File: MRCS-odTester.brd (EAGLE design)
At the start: 50 x 50 mm, 14 parts

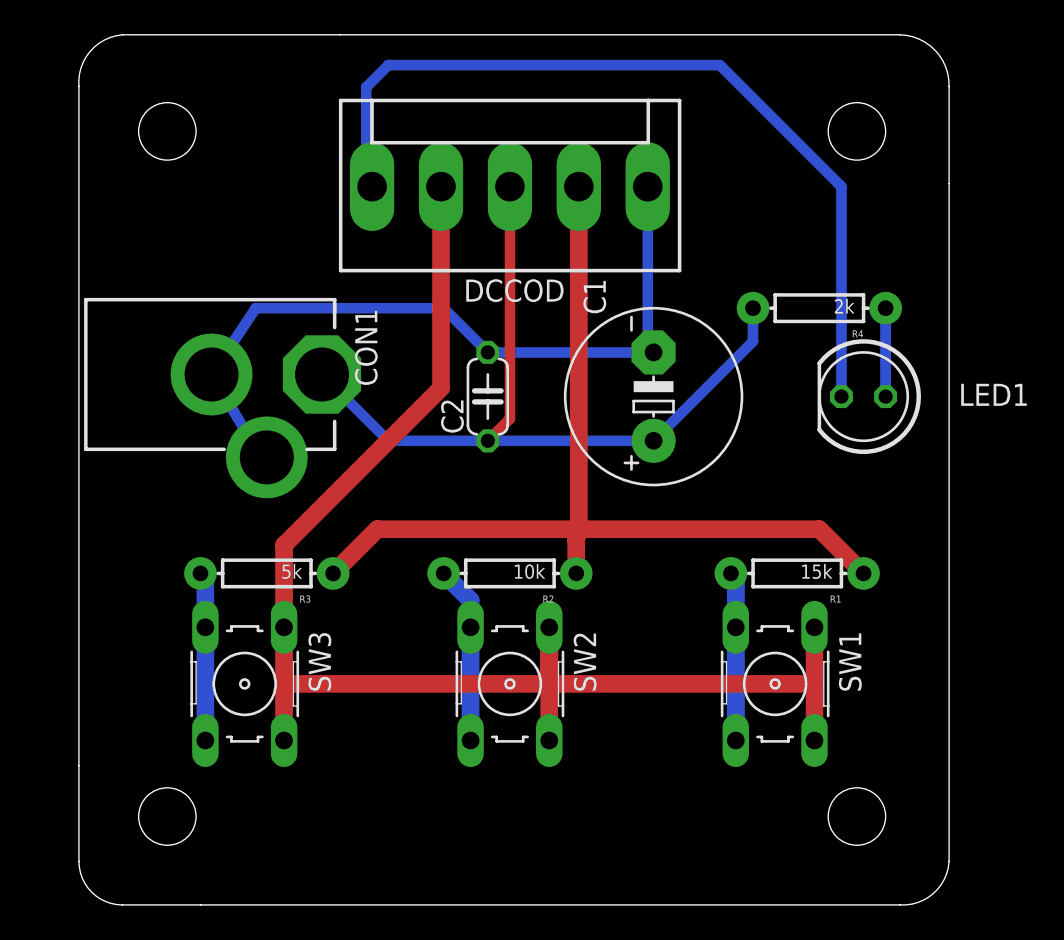
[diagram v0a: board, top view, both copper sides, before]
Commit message: 1.1
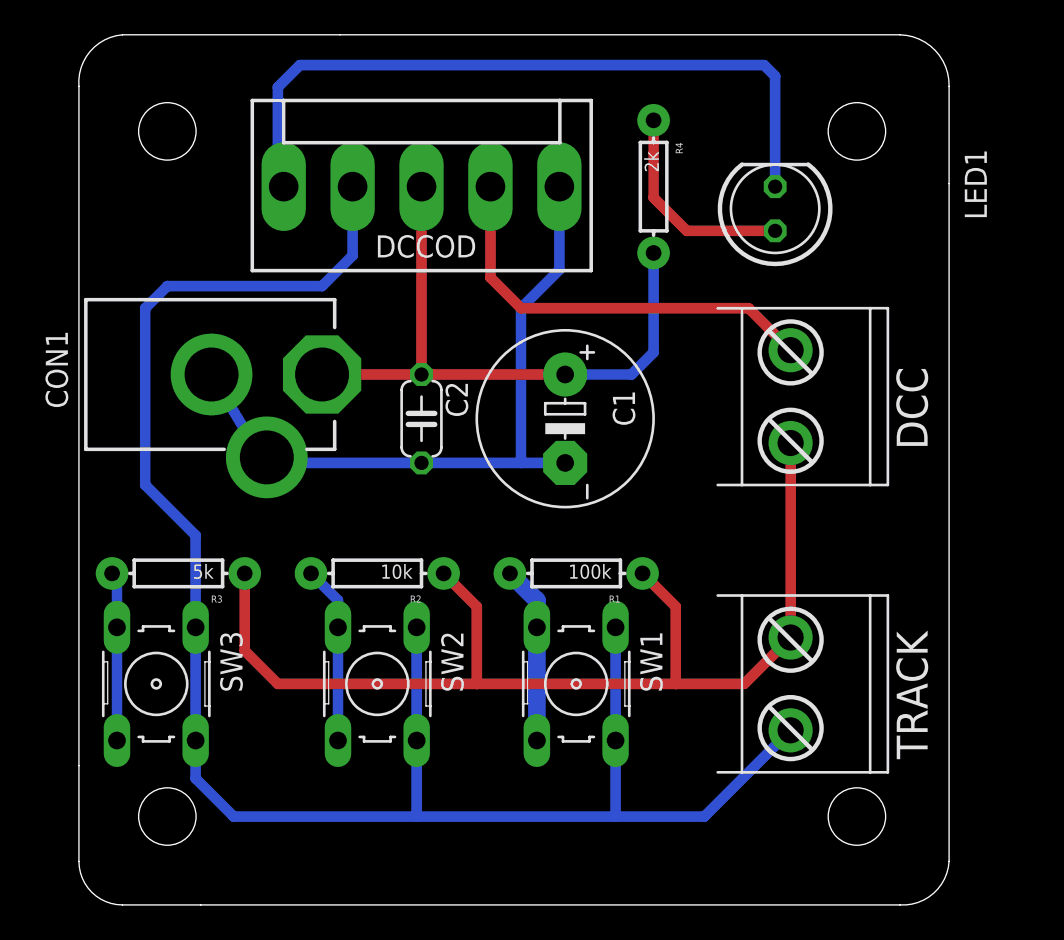
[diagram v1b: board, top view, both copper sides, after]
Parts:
- added DCC, TRACK: (no value), SPCoast:MSTB2
- R1: value 15k -> 100k
- moved R1 12.7 mm to (28.6, 19.1)
- moved LED1 11.9 mm to (40.0, 40.0), turned to 90 degrees
- moved R4 11.8 mm to (33.0, 41.3), turned to 270 degrees
- moved SW1 11.4 mm to (28.6, 12.7)
- moved R2 7.62 mm to (17.1, 19.1)
- moved SW2 7.62 mm to (17.1, 12.7)
- moved C1 5.24 mm to (27.9, 27.9), turned to 270 degrees
- moved DCCOD 5.08 mm to (19.7, 41.3)
- moved R3 5.08 mm to (5.71, 19.1)
- moved SW3 5.08 mm to (4.45, 12.7)
- moved C2 4.02 mm to (19.7, 27.9), turned to 270 degrees
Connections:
- removed net TRACK+: DCCOD.2, SW1.1, SW1.2, SW2.1, SW2.2, SW3.1, SW3.2
- removed net TRACK-: DCCOD.4, R1.P$1, R2.P$1, R3.P$1
- new net DCC-COMMON: DCC.2, DCCOD.4
- new net DCC-FROMTRACK: DCCOD.2, SW1.1, SW1.2, SW2.1, SW2.2, SW3.1, SW3.2, TRACK.1
- new net DCC-TOTRACK: DCC.1, R1.P$1, R2.P$1, R3.P$1, TRACK.2
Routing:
- net DCC-FROMTRACK: track 0.00 -> 104.2 mm
- net TRACK+: track 82.3 -> 0.00 mm
- net DCC-TOTRACK: track 0.00 -> 63.2 mm
- net TRACK-: track 55.5 -> 0.00 mm
- net DCC-COMMON: track 0.00 -> 24.2 mm
- net +12V: track 45.7 -> 36.1 mm
- net N$5: track 5.08 -> 12.2 mm
- net VOUT: track 48.6 -> 41.6 mm
- net GND: track 43.8 -> 40.0 mm
- net N$1: track 9.72 -> 10.2 mm
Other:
- board text added: ""Too Low" and "Normal" lights mean Normal"
- board text added: "Adjust for Normal Detection and not "Too High""
- board text added: "DCCOD"
- board text added: "DCCOD Tester"
- board text added: "Go Bears!"
- board text added: "If all three light, the detector is too sensitive"
- board text added: "If only "too low" lights, the detector is not sensitive enough"
- board text added: "Made in the PCR, Coast Div, NMRA"
- board text added: "Model Railroading is Fun!"
- board text added: "Test"
- board text added: "Too HIGH"
- board text added: "Too LOW"
- board text added: "www.SPCoast.com"
- board text removed: "HIGH"
- board text removed: "LOW"
- board text removed: "Sensitivity"
